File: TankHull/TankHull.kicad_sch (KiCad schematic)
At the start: 80 parts, among them J1 SlipRing_4, J2 Conn_01x02_Socket, J3 Conn_01x02_Socket, J4 Conn_01x02_Socket, J5 Conn_01x02_Socket, J7 Conn_01x05, Q1 Q_PMOS, U10 IRM-V838M3-C/TR1, U11 IRM-V838M3-C/TR1, U12 IRM-V838M3-C/TR1, U2 DRV8833PWP, U3 DRV8833PWP, U4 IRM-V838M3-C/TR1, U5 IRM-V838M3-C/TR1, U6 IRM-V838M3-C/TR1, U7 IRM-V838M3-C/TR1, U8 PCA9555PW, U9 IRM-V838M3-C/TR1

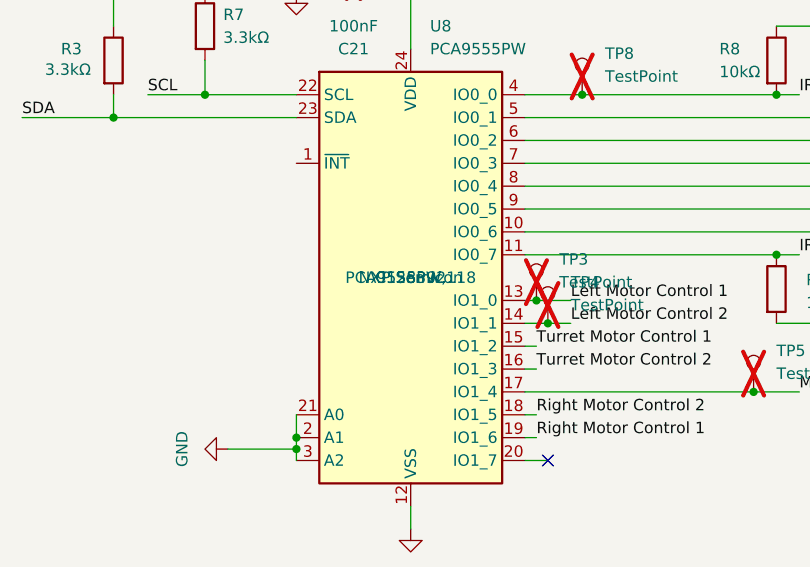
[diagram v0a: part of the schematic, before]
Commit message: bits
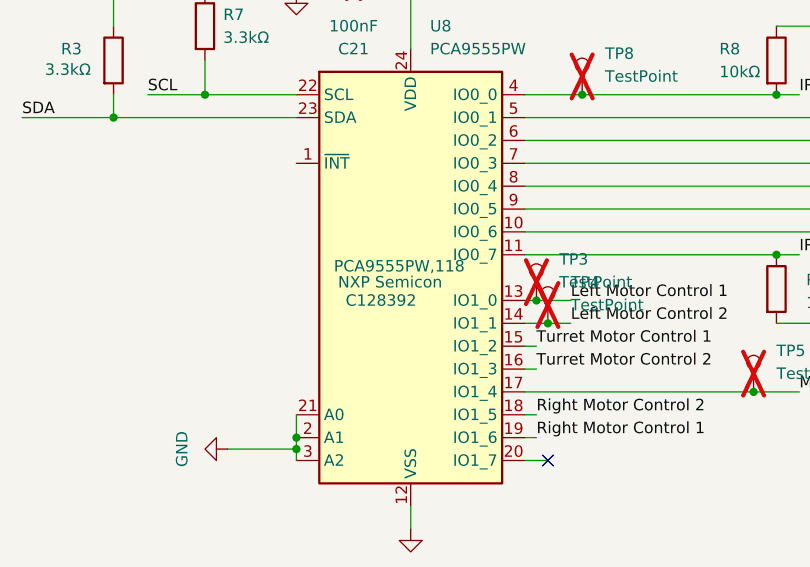
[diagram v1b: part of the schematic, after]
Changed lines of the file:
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@@
 		(on_board yes)
 		(dnp no)
-		(fields_autoplaced yes)
 		(property "Reference" "U8"
 			(at 91.0433 115.57 0)
@@
 		)
 		(property "JLCPCB Part #" "C128392"
-			(at 88.9 143.51 0)
+			(at 85.598 146.05 0)
 			(effects
 				(font
@@
 		)
 		(property "MANUFACTURER" "NXP Semicon "
-			(at 88.9 143.51 0)
+			(at 86.614 144.018 0)
 			(effects
 				(font
@@
 		)
 		(property "Manufacturer_Part_Number" "PCA9555PW,118"
-			(at 88.9 143.51 0)
+			(at 87.63 142.24 0)
 			(effects
 				(font
